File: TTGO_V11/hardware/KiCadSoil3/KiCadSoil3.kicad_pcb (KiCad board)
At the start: 2 copper layers, 83.8 x 19.7 mm, 12 parts, among them J1 Screw_Terminal_01x03, U1 ATtiny85, U2 TLC555CP, U3 DS18B20

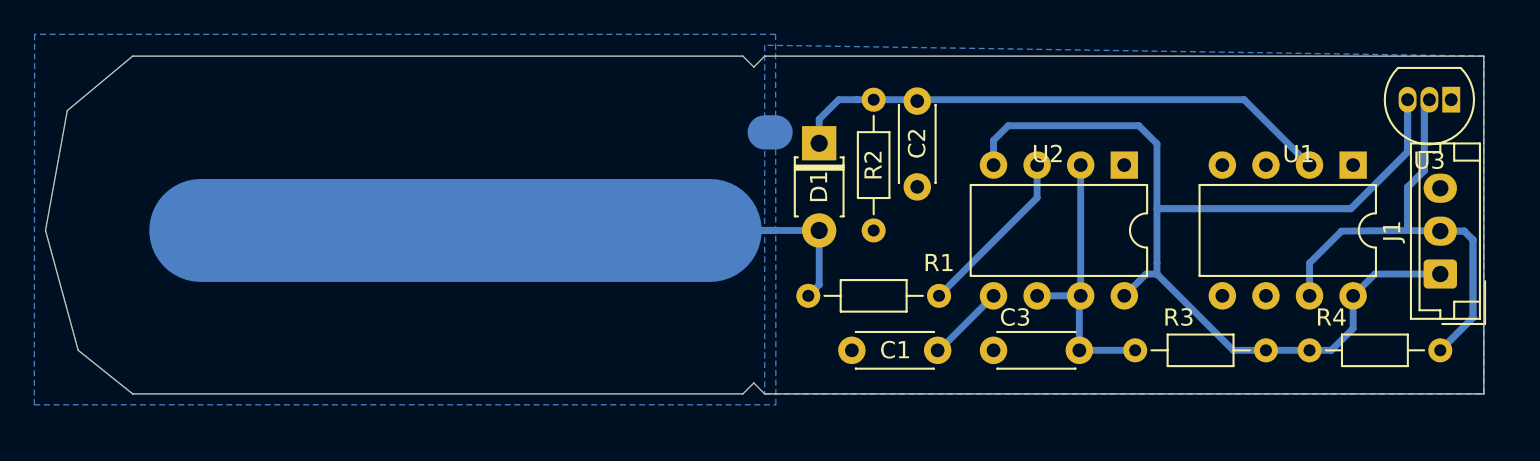
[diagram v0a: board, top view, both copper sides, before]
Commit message: changes
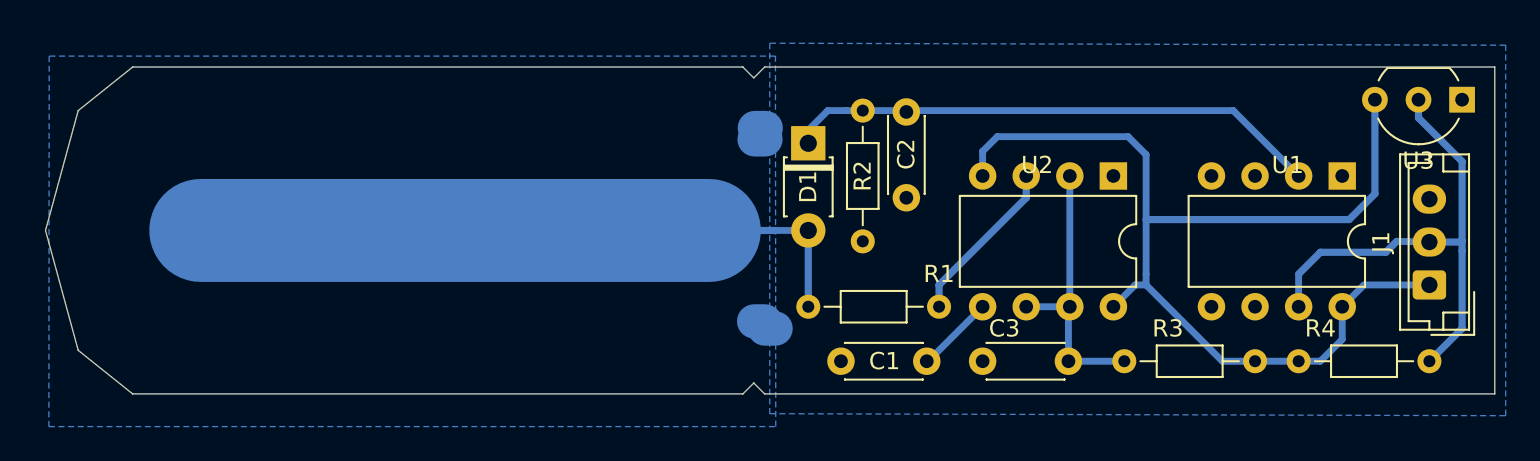
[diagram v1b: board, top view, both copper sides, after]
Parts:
- U1: value ATtiny85 -> ATtiny85-20PU
- U3: footprint Package_TO_SOT_THT:TO-92_Inline -> Package_TO_SOT_THT:TO-92_Inline_Wide
- moved C1 0.90 mm to (76.8, 48.9)
- moved J1 0.90 mm to (111.1, 44.5)
- moved R4 0.90 mm to (103.5, 48.9)
- moved C2 0.90 mm to (80.6, 39.4)
- moved U1 0.90 mm to (106.0, 38.1)
- moved U2 0.90 mm to (92.7, 38.1)
- moved C3 0.90 mm to (85.1, 48.9)
- moved R3 0.90 mm to (101.0, 48.9)
- moved R2 0.90 mm to (78.1, 41.9)
- moved U3 0.64 mm to (113.0, 33.7)
- moved R1 0.63 mm to (74.9, 45.7)
- moved D1 0.63 mm to (74.9, 36.2)
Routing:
- net GND: track 0.64 -> 2.54 mm
- net /1-Wire: track 27.8 -> 29.3 mm
- net /AOUT: track 32.1 -> 30.7 mm
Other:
- board size 83.8 x 19.7 mm -> 84.5 x 19 mm
